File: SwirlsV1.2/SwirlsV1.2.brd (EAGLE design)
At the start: 38.7 x 106.8 mm, 130 parts, among them IC1 LM1117-3.3, IC2 LM4040B25, IC3 LM1117-3.3, IC4 DAC8552, IC5 TL072, IC6 TL072, IC7 LM4040B10, IC8 MCP6002, IC9 MCP6004, J1 PJ301_GUI6, J10 PJ301_GUI6, J11 PJ301_GUI6, J12 PJ301_GUI6, J13 PJ301_GUI6, J2 PJ301_GUI6, J3 PJ301_GUI6, J4 PJ301_GUI6, J5 PJ301_GUI6, J6 PJ301_GUI6, J7 PJ301_GUI6, J8 PJ301_GUI6, J9 PJ301_GUI6, Q1 8MHz, Q2 MMBT3904, Q3 MMBT3904, Q4 MMBT3904, Q5 MMBT3904, Q6 MMBT3904, SW3 TL1100X, SW4 TL1100X

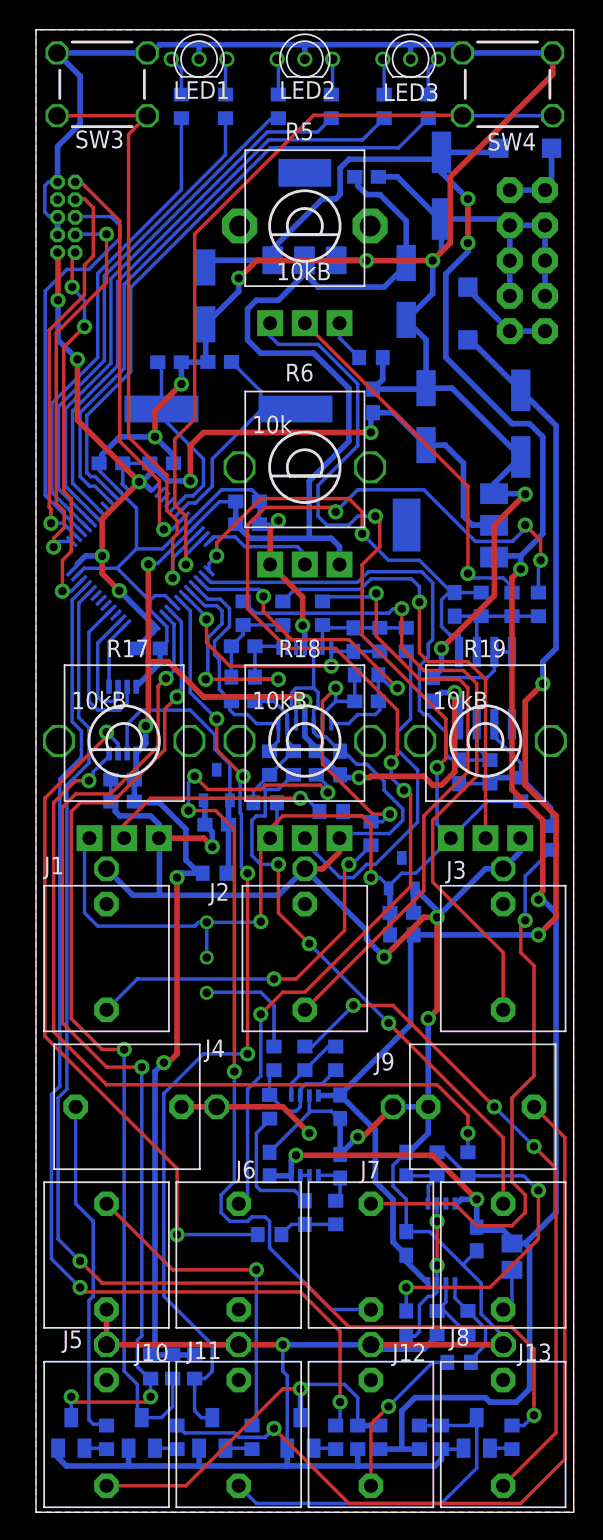
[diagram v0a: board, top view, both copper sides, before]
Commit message: fixed
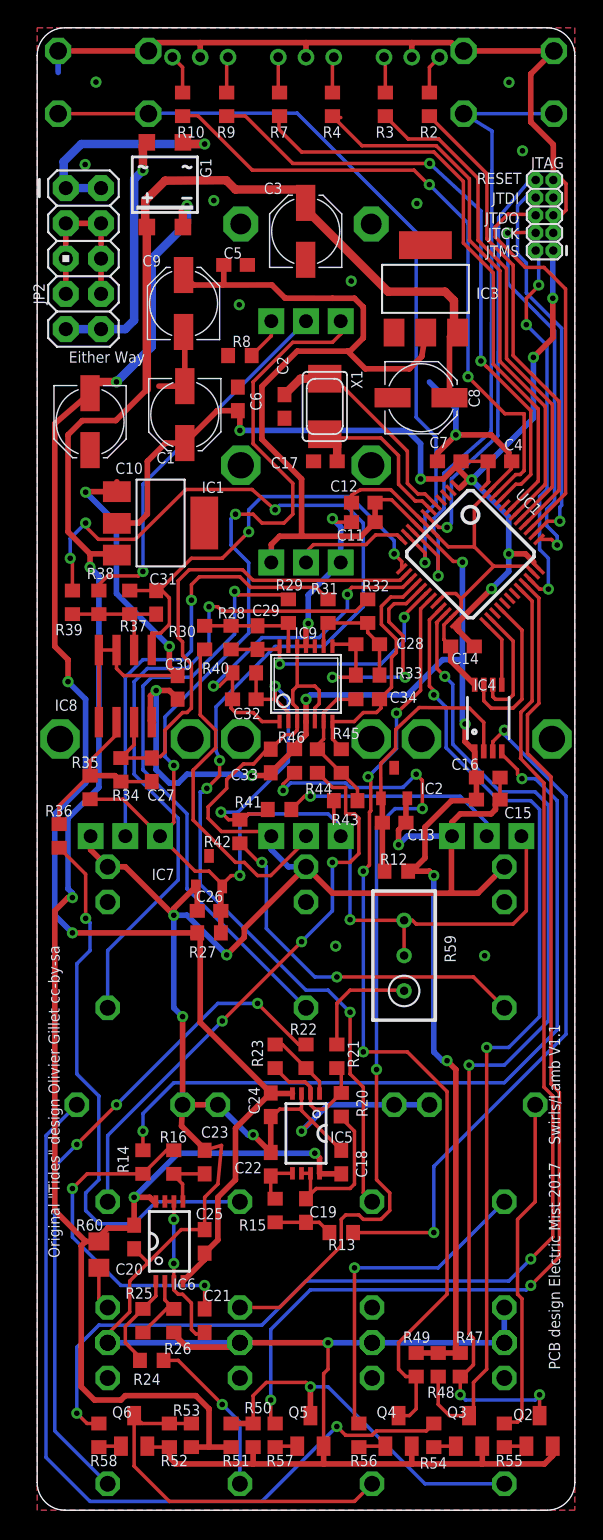
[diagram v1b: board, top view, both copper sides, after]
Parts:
- removed D1, D2: 1N5819HW, diode:SOD123
- removed POWER: M05X2PTH, og-header:AVR_ICSP
- removed Q1: 8MHz, SparkFun-Clocks:HC49UP
- added G1: (no value), microbuilder:SOIC-4
- added JP2: M05X2PTH, braids_v50:AVR_ICSP
- added X1: (no value), Icotech_Eagle_Library:NX5032
- C10, C3: device rcl:PANASONIC_D -> rcl:PANASONIC_C
- R6: value 10k -> 10kb
- moved R36 35.5 mm to (1.67, 48.7), flipped to the top
- moved Q2 33.7 mm to (36.3, 5.86), flipped to the top
- moved R39 33.6 mm to (2.62, 65.6), flipped to the top
- moved JTAG 33.2 mm to (36.0, 94.7), flipped to the top
- moved C10 31.0 mm to (3.89, 78.6), flipped to the top
- moved R35 31.0 mm to (3.89, 52.2), flipped to the top
- moved R38 29.8 mm to (4.53, 65.6), flipped to the top
- moved R58 29.8 mm to (4.53, 5.54), flipped to the top
- moved R60 29.8 mm to (4.53, 18.6), flipped to the top
- moved SW3 29.3 mm to (34.1, 103.0), flipped to the bottom
- moved SW4 29.1 mm to (4.85, 103.0), flipped to the bottom
- moved J1 28.7 mm to (33.7, 40.8), flipped to the bottom
- moved J10 28.7 mm to (33.7, 6.50), flipped to the bottom
- moved J5 28.7 mm to (33.7, 17.9), flipped to the bottom
- moved R55 28.7 mm to (33.7, 5.54), flipped to the top
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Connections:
- removed net N$56: D1.A, POWER.1, POWER.2
- removed net N$64: D2.C, POWER.10, POWER.9
- new net N$49: G1.~1, JP2.1, JP2.2
- new net N$50: G1.~2, JP2.10, JP2.9
- net GND: now also JP2.3, JP2.4, JP2.5, JP2.6, JP2.7, JP2.8; no longer POWER.3, POWER.4, POWER.5, POWER.6, POWER.7, POWER.8
- net N$7: now also X1.P$2; no longer Q1.2
- net N$8: now also X1.P$1; no longer Q1.1
- net VCC: now also G1.+; no longer D1.C
- net VEE: now also G1.-; no longer D2.A
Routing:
- net GND: track 491.5 -> 411.9 mm, vias 16 -> 22
- net N$50: track 0.00 -> 18.4 mm, vias 0 -> 1
- net N$49: track 0.00 -> 16.9 mm, vias 0 -> 1
- net VEE: track 88.9 -> 102.2 mm, vias 2 -> 4
- net N$64: track 6.96 -> 0.00 mm
- net N$56: track 5.75 -> 0.00 mm
- net VCC: track 168.4 -> 172.1 mm, vias 6 -> 4
- net N$8: track 16.9 -> 13.3 mm
- net N$36: track 39.1 -> 42.6 mm
- net N$37: track 36.3 -> 39.8 mm
- net N$7: track 13.6 -> 16.7 mm
- net N$34: track 44.1 -> 47.1 mm, vias 0 -> 2
- net N$35: track 41.8 -> 44.6 mm, vias 0 -> 2
- net N$38: track 35.0 -> 36.3 mm
- net CYCLE_SW: track 46.1 -> 47.0 mm
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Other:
- outline, holes or cut-outs redrawn
- board text added: "Either Way"
- board text removed: "-12V"
